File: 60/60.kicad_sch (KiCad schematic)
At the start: 24 parts, among them J1 AVR-ISP-6, J2 78171-0004, J3 TYPE-C-31-M-12, SW2 SW_Push_Reset, U1 ATmega32U4-A, Y1 16MHz

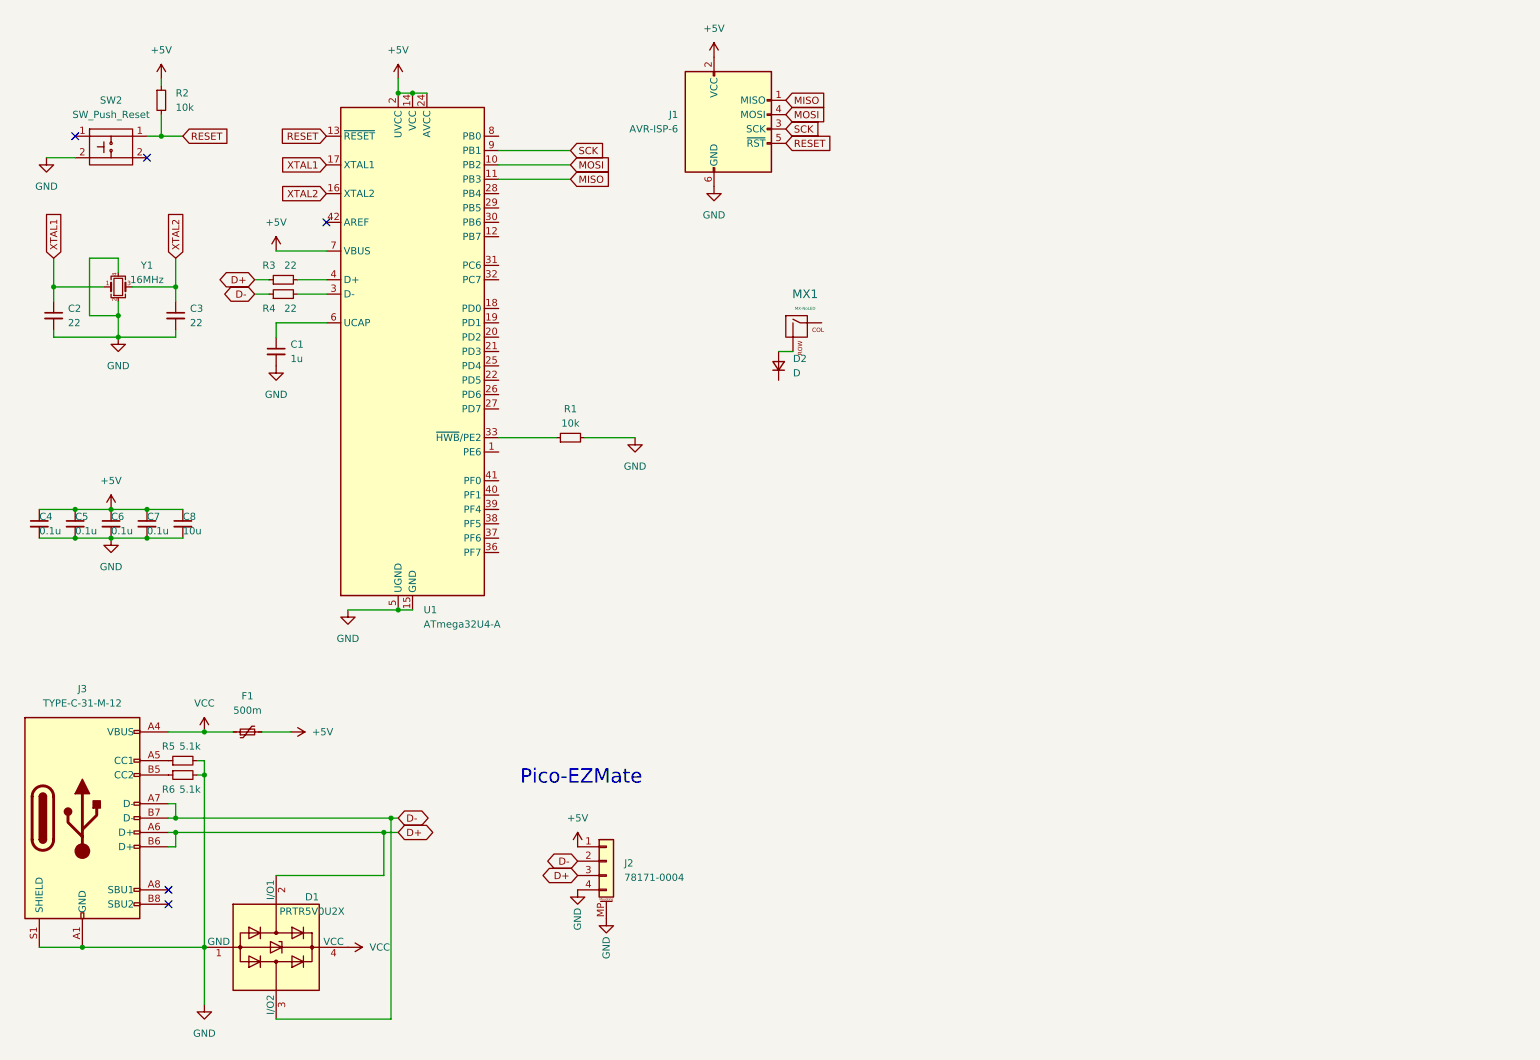
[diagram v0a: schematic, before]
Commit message: Initialize the matrix
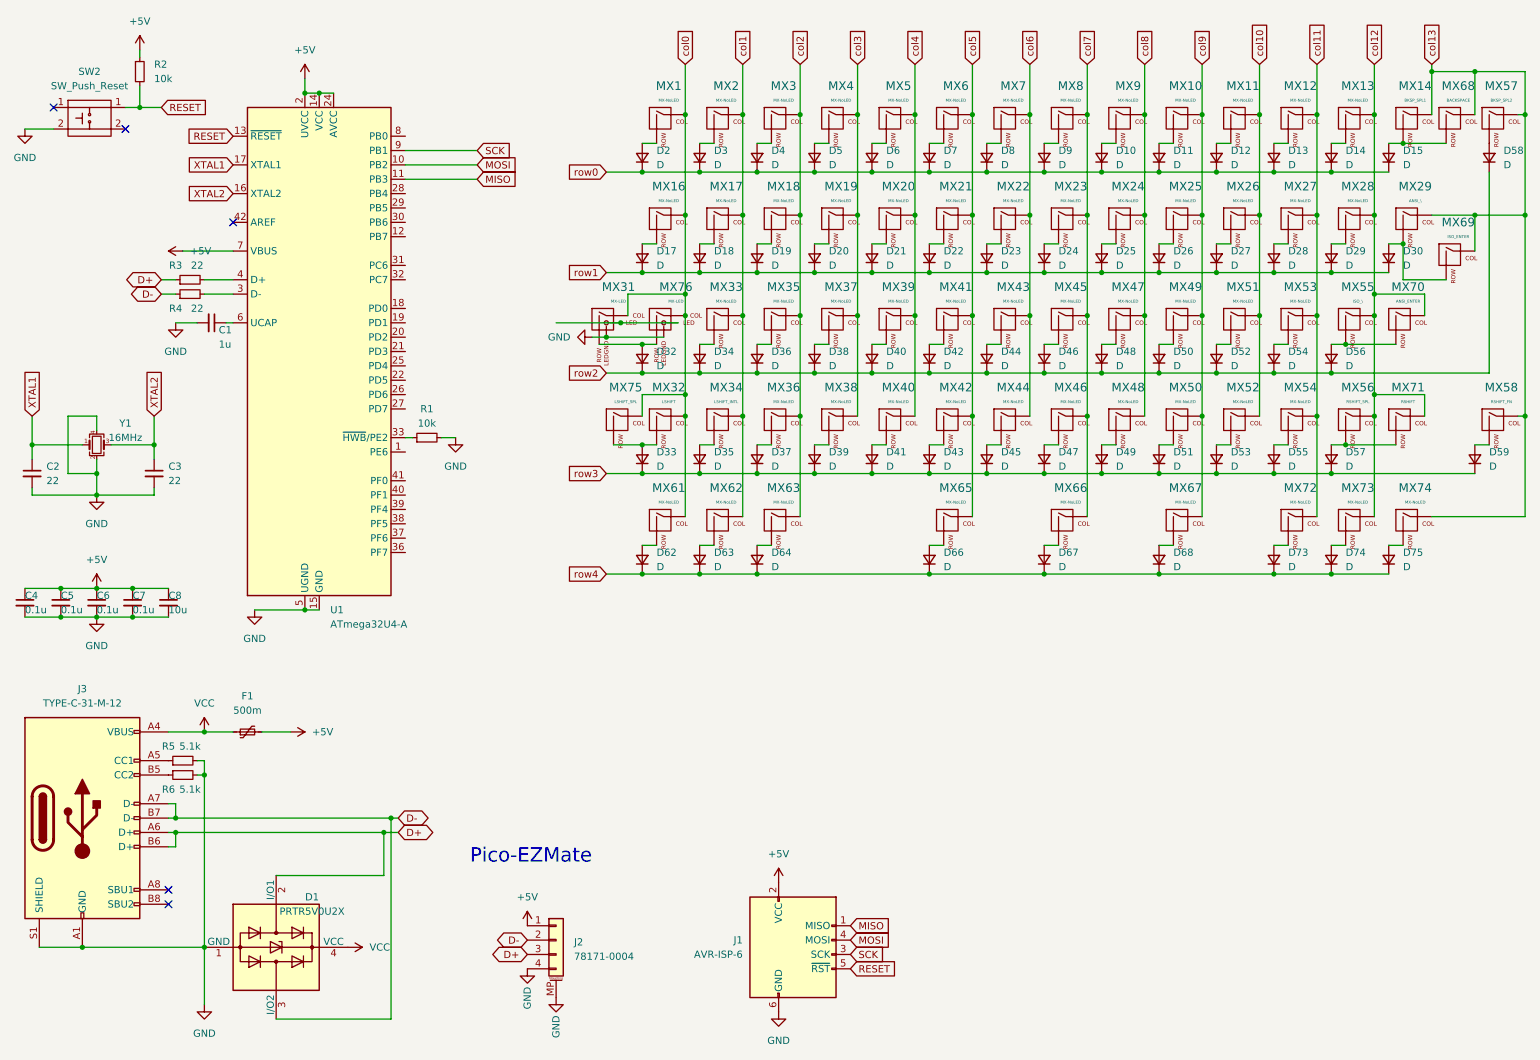
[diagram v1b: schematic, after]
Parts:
- added D10, D11, D12, D13, D14, D15, D17, D18, D19, D20, D21, D22, D23, D24, D25, D26, D27, D28, D29, D3, D30, D32, D33, D34, D35, D36, D37, D38, D39, D4, D40, D41, D42, D43, D44, D45, D46, D47, D48, D49, D5, D50, D51, D52, D53, D54, D55, D56, D57, D58, D59, D6, D62, D63, D64, D66, D67, D68, D7, D73, D74, D75, D8, D9: D, symbol Device:D_Small
- added MX10, MX11, MX12, MX13, MX16, MX17, MX18, MX19, MX2, MX20, MX21, MX22, MX23, MX24, MX25, MX26, MX27, MX28, MX3, MX33, MX35, MX36, MX37, MX38, MX39, MX4, MX40, MX41, MX42, MX43, MX44, MX45, MX46, MX47, MX48, MX49, MX5, MX50, MX51, MX52, MX53, MX54, MX6, MX61, MX62, MX63, MX65, MX66, MX67, MX7, MX72, MX73, MX74, MX8, MX9: MX-NoLED, symbol MX_Alps_Hybrid:MX-NoLED
- added MX14: BKSP_SPL1, symbol MX_Alps_Hybrid:MX-NoLED
- added MX29: ANSI_\, symbol MX_Alps_Hybrid:MX-NoLED
- added MX31, MX76: MX-LED, symbol MX_Alps_Hybrid:MX-LED
- added MX32: LSHIFT, symbol MX_Alps_Hybrid:MX-NoLED
- added MX34: LSHIFT_INTL, symbol MX_Alps_Hybrid:MX-NoLED
- added MX55: ISO_\, symbol MX_Alps_Hybrid:MX-NoLED
- added MX56: RSHIFT_SPL, symbol MX_Alps_Hybrid:MX-NoLED
- added MX57: BKSP_SPL2, symbol MX_Alps_Hybrid:MX-NoLED
- added MX58: RSHIFT_FN, symbol MX_Alps_Hybrid:MX-NoLED
- added MX68: BACKSPACE, symbol MX_Alps_Hybrid:MX-NoLED
- added MX69: ISO_ENTER, symbol MX_Alps_Hybrid:MX-NoLED
- added MX70: ANSI_ENTER, symbol MX_Alps_Hybrid:MX-NoLED
- added MX71: RSHIFT, symbol MX_Alps_Hybrid:MX-NoLED
- added MX75: LSHIFT_SPL, symbol MX_Alps_Hybrid:MX-NoLED
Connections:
- net GND: now also MX31.4 (LEDGND), MX76.4 (LEDGND)
- net row0: now reaches D2.1 (K)
- net row0: now also D10.1 (K), D11.1 (K), D12.1 (K), D13.1 (K), D14.1 (K), D15.1 (K), D3.1 (K), D4.1 (K), D5.1 (K), D6.1 (K), D7.1 (K), D8.1 (K), D9.1 (K)
- net col0: now reaches MX1.1 (COL)
- net col0: now also MX16.1 (COL), MX31.1 (COL), MX32.1 (COL), MX61.1 (COL), MX75.1 (COL), MX76.1 (COL)
- new net: D56.2 (A), MX55.2 (ROW), MX70.2 (ROW)
- new net: D46.2 (A), MX45.2 (ROW)
- new net: D4.2 (A), MX3.2 (ROW)
- new net: D29.2 (A), MX28.2 (ROW)
- new net: D8.2 (A), MX7.2 (ROW)
- new net: D44.2 (A), MX43.2 (ROW)
- new net: D39.2 (A), MX38.2 (ROW)
- new net: D5.2 (A), MX4.2 (ROW)
- new net: D11.2 (A), MX10.2 (ROW)
- new net: D30.2 (A), MX29.2 (ROW), MX69.2 (ROW)
- new net: D62.2 (A), MX61.2 (ROW)
- new net: D43.2 (A), MX42.2 (ROW)
- new net: D51.2 (A), MX50.2 (ROW)
- new net: D55.2 (A), MX54.2 (ROW)
- new net: D57.2 (A), MX56.2 (ROW), MX71.2 (ROW)
- new net: D66.2 (A), MX65.2 (ROW)
- new net: D35.2 (A), MX34.2 (ROW)
- new net: D48.2 (A), MX47.2 (ROW)
- new net: D14.2 (A), MX13.2 (ROW)
- new net: D67.2 (A), MX66.2 (ROW)
- new net: D41.2 (A), MX40.2 (ROW)
- new net: D73.2 (A), MX72.2 (ROW)
- new net: D49.2 (A), MX48.2 (ROW)
- new net: D23.2 (A), MX22.2 (ROW)
- new net: D21.2 (A), MX20.2 (ROW)
- new net: D68.2 (A), MX67.2 (ROW)
- new net: D24.2 (A), MX23.2 (ROW)
- new net: D10.2 (A), MX9.2 (ROW)
- new net: D74.2 (A), MX73.2 (ROW)
- new net: D40.2 (A), MX39.2 (ROW)
- new net: D47.2 (A), MX46.2 (ROW)
- new net: D50.2 (A), MX49.2 (ROW)
- new net: D63.2 (A), MX62.2 (ROW)
- new net: D13.2 (A), MX12.2 (ROW)
- new net: D7.2 (A), MX6.2 (ROW)
- new net: D53.2 (A), MX52.2 (ROW)
- new net: D34.2 (A), MX33.2 (ROW)
- new net: D19.2 (A), MX18.2 (ROW)
- new net: D37.2 (A), MX36.2 (ROW)
- new net: D18.2 (A), MX17.2 (ROW)
- new net: D6.2 (A), MX5.2 (ROW)
- new net: D33.2 (A), MX32.2 (ROW), MX75.2 (ROW)
- new net: D58.2 (A), MX57.2 (ROW)
- new net: D64.2 (A), MX63.2 (ROW)
- new net: D9.2 (A), MX8.2 (ROW)
- new net: D75.2 (A), MX74.2 (ROW)
- new net: D17.2 (A), MX16.2 (ROW)
- new net: D25.2 (A), MX24.2 (ROW)
- new net: D38.2 (A), MX37.2 (ROW)
- new net: D12.2 (A), MX11.2 (ROW)
- new net: D22.2 (A), MX21.2 (ROW)
- new net: D27.2 (A), MX26.2 (ROW)
- new net: D28.2 (A), MX27.2 (ROW)
- new net: D45.2 (A), MX44.2 (ROW)
- new net: D15.2 (A), MX14.2 (ROW), MX68.2 (ROW)
- new net: D54.2 (A), MX53.2 (ROW)
- new net: D3.2 (A), MX2.2 (ROW)
- new net: D36.2 (A), MX35.2 (ROW)
- new net: D42.2 (A), MX41.2 (ROW)
- new net: D59.2 (A), MX58.2 (ROW)
- new net: D32.2 (A), MX31.2 (ROW), MX76.2 (ROW)
- new net: D20.2 (A), MX19.2 (ROW)
- new net: D26.2 (A), MX25.2 (ROW)
- new net: MX31.3 (LED), MX76.3 (LED)
- new net: D52.2 (A), MX51.2 (ROW)
- new net col1: MX17.1 (COL), MX2.1 (COL), MX33.1 (COL), MX34.1 (COL), MX62.1 (COL)
- new net col10: MX11.1 (COL), MX26.1 (COL), MX51.1 (COL), MX52.1 (COL)
- new net col11: MX12.1 (COL), MX27.1 (COL), MX53.1 (COL), MX54.1 (COL), MX72.1 (COL)
- new net col12: MX13.1 (COL), MX28.1 (COL), MX55.1 (COL), MX56.1 (COL), MX70.1 (COL), MX71.1 (COL), MX73.1 (COL)
- new net col13: MX14.1 (COL), MX29.1 (COL), MX57.1 (COL), MX58.1 (COL), MX68.1 (COL), MX69.1 (COL), MX74.1 (COL)
- new net col2: MX18.1 (COL), MX3.1 (COL), MX35.1 (COL), MX36.1 (COL), MX63.1 (COL)
- new net col3: MX19.1 (COL), MX37.1 (COL), MX38.1 (COL), MX4.1 (COL)
- new net col4: MX20.1 (COL), MX39.1 (COL), MX40.1 (COL), MX5.1 (COL)
- new net col5: MX21.1 (COL), MX41.1 (COL), MX42.1 (COL), MX6.1 (COL), MX65.1 (COL)
- new net col6: MX22.1 (COL), MX43.1 (COL), MX44.1 (COL), MX7.1 (COL)
- new net col7: MX23.1 (COL), MX45.1 (COL), MX46.1 (COL), MX66.1 (COL), MX8.1 (COL)
- new net col8: MX24.1 (COL), MX47.1 (COL), MX48.1 (COL), MX9.1 (COL)
- new net col9: MX10.1 (COL), MX25.1 (COL), MX49.1 (COL), MX50.1 (COL), MX67.1 (COL)
- new net row1: D17.1 (K), D18.1 (K), D19.1 (K), D20.1 (K), D21.1 (K), D22.1 (K), D23.1 (K), D24.1 (K), D25.1 (K), D26.1 (K), D27.1 (K), D28.1 (K), D29.1 (K), D30.1 (K)
- new net row2: D32.1 (K), D34.1 (K), D36.1 (K), D38.1 (K), D40.1 (K), D42.1 (K), D44.1 (K), D46.1 (K), D48.1 (K), D50.1 (K), D52.1 (K), D54.1 (K), D56.1 (K), D58.1 (K)
- new net row3: D33.1 (K), D35.1 (K), D37.1 (K), D39.1 (K), D41.1 (K), D43.1 (K), D45.1 (K), D47.1 (K), D49.1 (K), D51.1 (K), D53.1 (K), D55.1 (K), D57.1 (K), D59.1 (K)
- new net row4: D62.1 (K), D63.1 (K), D64.1 (K), D66.1 (K), D67.1 (K), D68.1 (K), D73.1 (K), D74.1 (K), D75.1 (K)
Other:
- moved on the sheet: C1, C2, C3, C4, C5, C6, C7, C8, D2, J1, J2, MX1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
